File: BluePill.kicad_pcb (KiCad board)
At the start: 2 copper layers, 91.9 x 73.2 mm, 91 parts, among them IC1 ADP2301AUJZ-R7, IC2 ADP2301AUJZ-R7, J1 SWD, J2 TE 338069-4, J3 Conn_02x08_Odd_Even, J4 BM04B-SURS-TFLFSN, J5 Conn_02x04_Odd_Even, J6 Conn_02x04_Odd_Even, J7 Conn_01x05, J8 Conn_01x02, J9 2169900003, Q1 AO3401A, SW1 SW_SPDT, U1 LM2842X, U2 STM32F405RGT6, U3 USBLC6-2SC6, U4 ICM-42670-P, U5 SN65HVD232QDRQ1, U6 XT30PW-F, U7 XT30PW-M, U8 LSF0102DCUR, Y1 16MHz

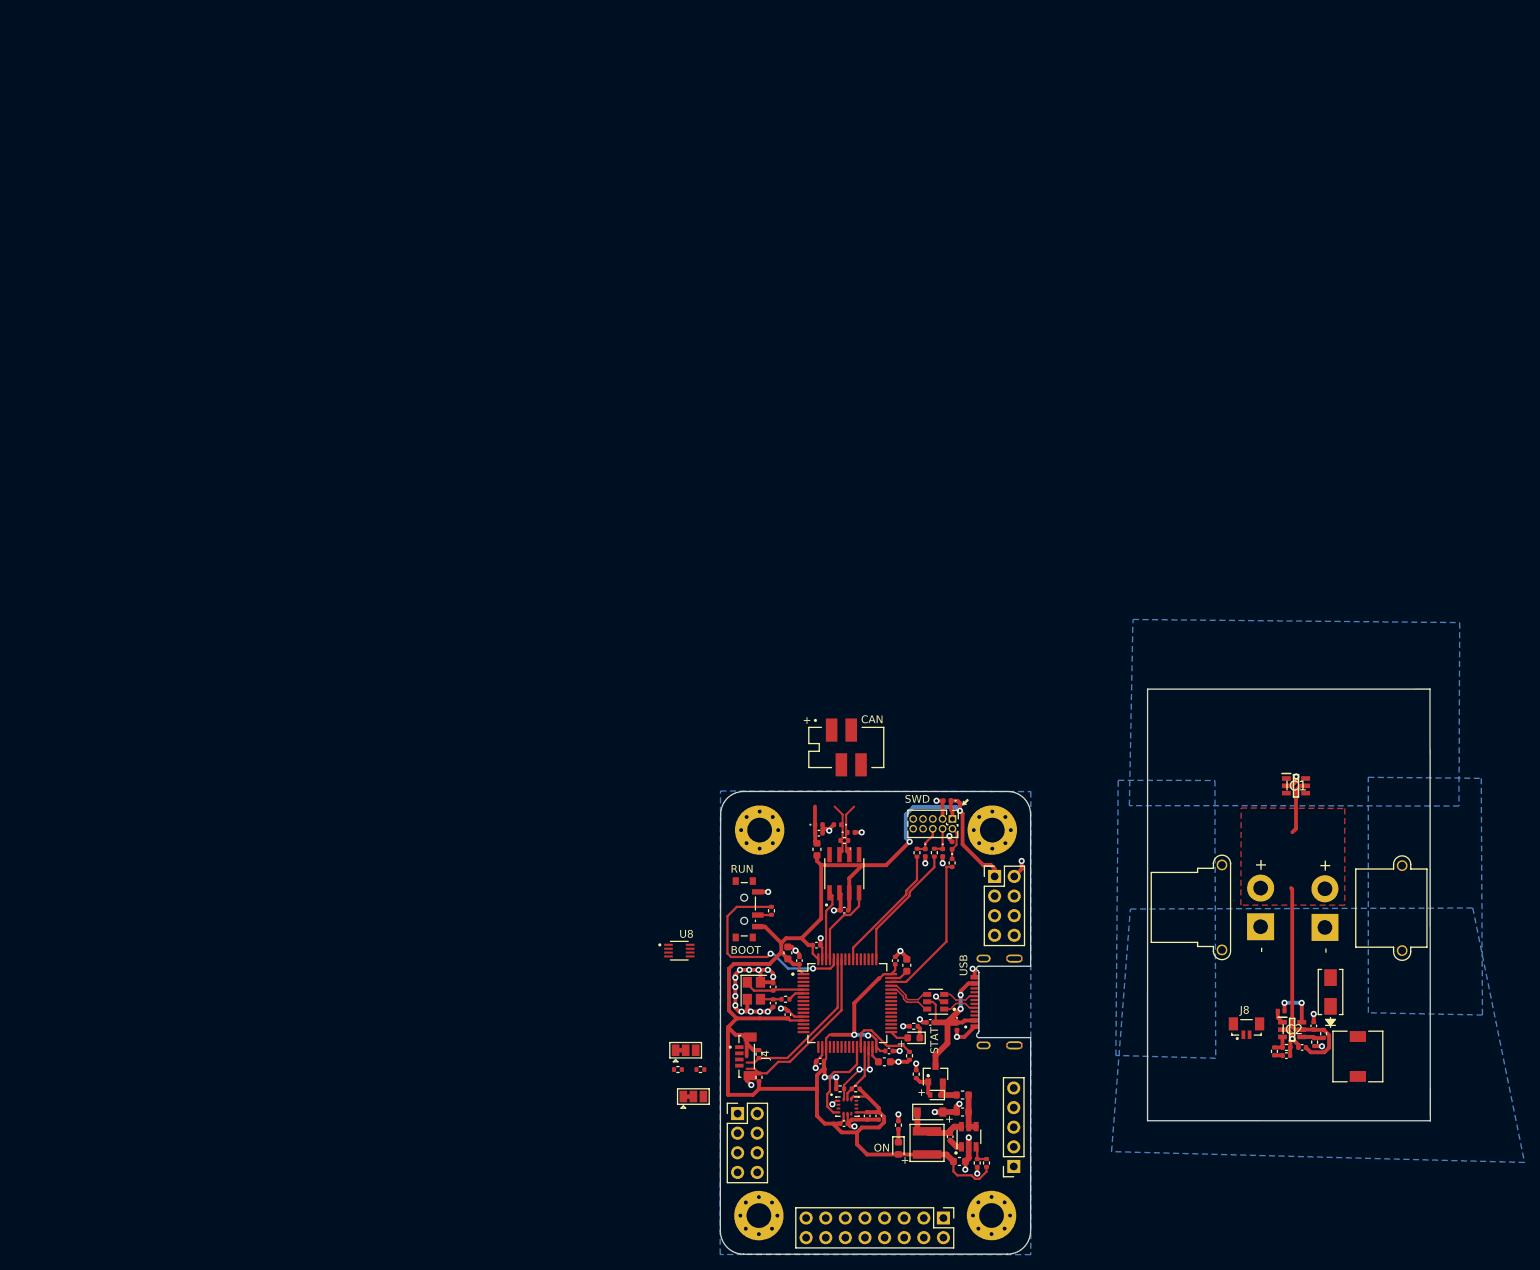
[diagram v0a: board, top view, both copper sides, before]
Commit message: skgnigniogni
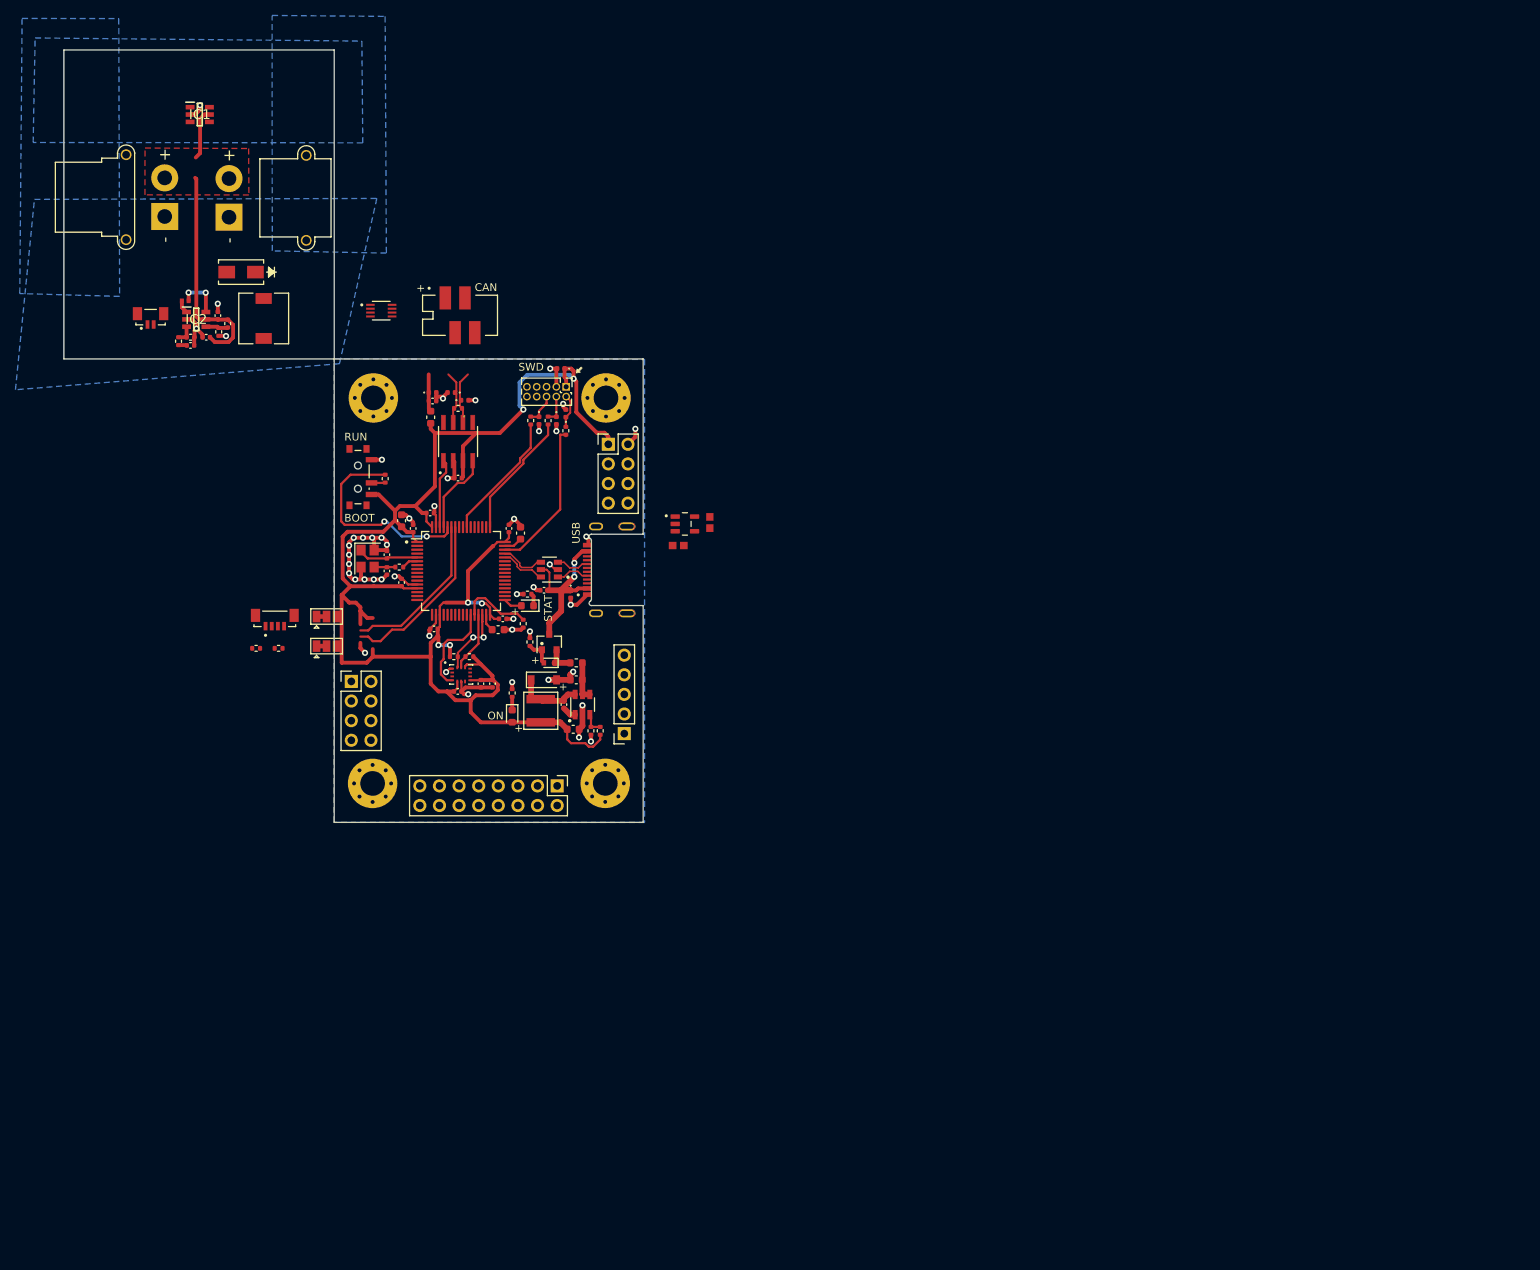
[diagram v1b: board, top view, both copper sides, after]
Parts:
- removed R11, R9: 2k2, Resistor_SMD:R_0402_1005Metric
- added C25: C0603C105K3RACTU, SnapEDA Library:C0603C105K3RACTU, F.Cu at (44.5, 24.2)
- added C26: C0603C105K3RACTU, SnapEDA Library:C0603C105K3RACTU, F.Cu at (48.6, 21.2)
- added U9: LP5907QMFX-3.3Q1, SnapEDA Library:SOT95P280X145-5N, F.Cu at (45.4, 21.4)
- moved L2 170.9 mm to (-9.13, -5.24)
- moved R20 169.1 mm to (-15.0, -3.50)
- moved C21 169.1 mm to (-15.1, -5.61)
- moved C22 169.1 mm to (-16.6, -2.81)
- moved C23 169.1 mm to (-19.3, -7.52)
- moved C24 169.1 mm to (-18.6, -1.75)
- moved IC2 169.1 mm to (-17.9, -5.12)
- moved J8 169.1 mm to (-23.8, -4.46)
- moved R19 169.1 mm to (-13.8, -4.58)
- moved R21 169.1 mm to (-20.2, -2.30)
- moved R22 169.1 mm to (-18.6, -2.81)
- moved U6 169.1 mm to (-21.9, -18.4)
- moved U7 169.1 mm to (-13.6, -18.4)
- moved D13 169.1 mm to (-12.1, -11.2), turned to 180 degrees
- moved IC1 166.4 mm to (-17.4, -31.6)
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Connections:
- U8 pad 1: unconnected-(U8-Pad1) -> GND
- U8 pad 2: unconnected-(U8-Pad2) -> +5V
- U8 pad 3: unconnected-(U8-Pad3) -> Servo_RXD
- U8 pad 4: unconnected-(U8-Pad4) -> Servo_TXD
- U8 pad 5: unconnected-(U8-Pad5) -> MCU_TXD
- U8 pad 6: unconnected-(U8-Pad6) -> MCU_RXD
- U8 pad 7: unconnected-(U8-Pad7) -> +3V3
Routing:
- net +3V3: track 233.9 -> 211.4 mm
- net MCU_I2C1_SCL: track 0.00 -> 22.5 mm
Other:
- board size 91.9 x 73.2 mm -> 75 x 100 mm
